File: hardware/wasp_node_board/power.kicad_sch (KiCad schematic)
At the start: 29 parts, among them J1 Conn_01x02, J7 USB_C_Receptacle_USB2.0_16P, SW1 C&K JS102011SAQN, U2 USBLC6-2SC6, U4 TPSM863253RDXR, U6 LP5907MFX-1.2

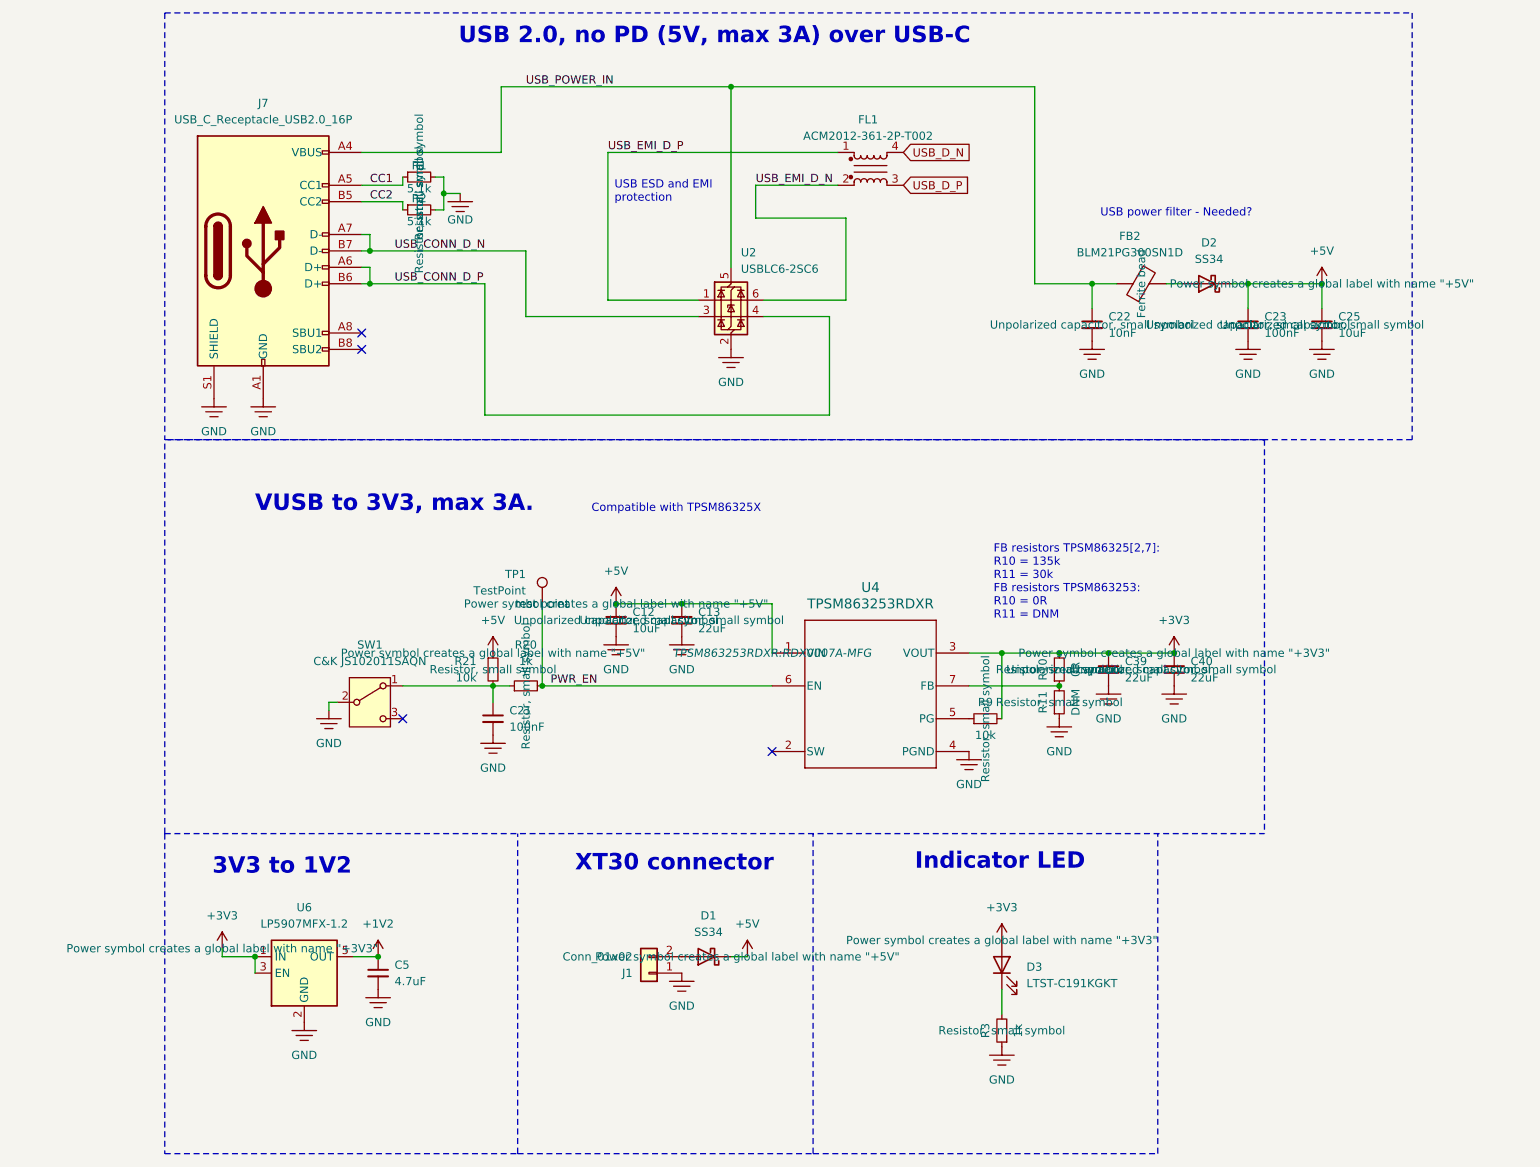
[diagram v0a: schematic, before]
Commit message: V1 layout done
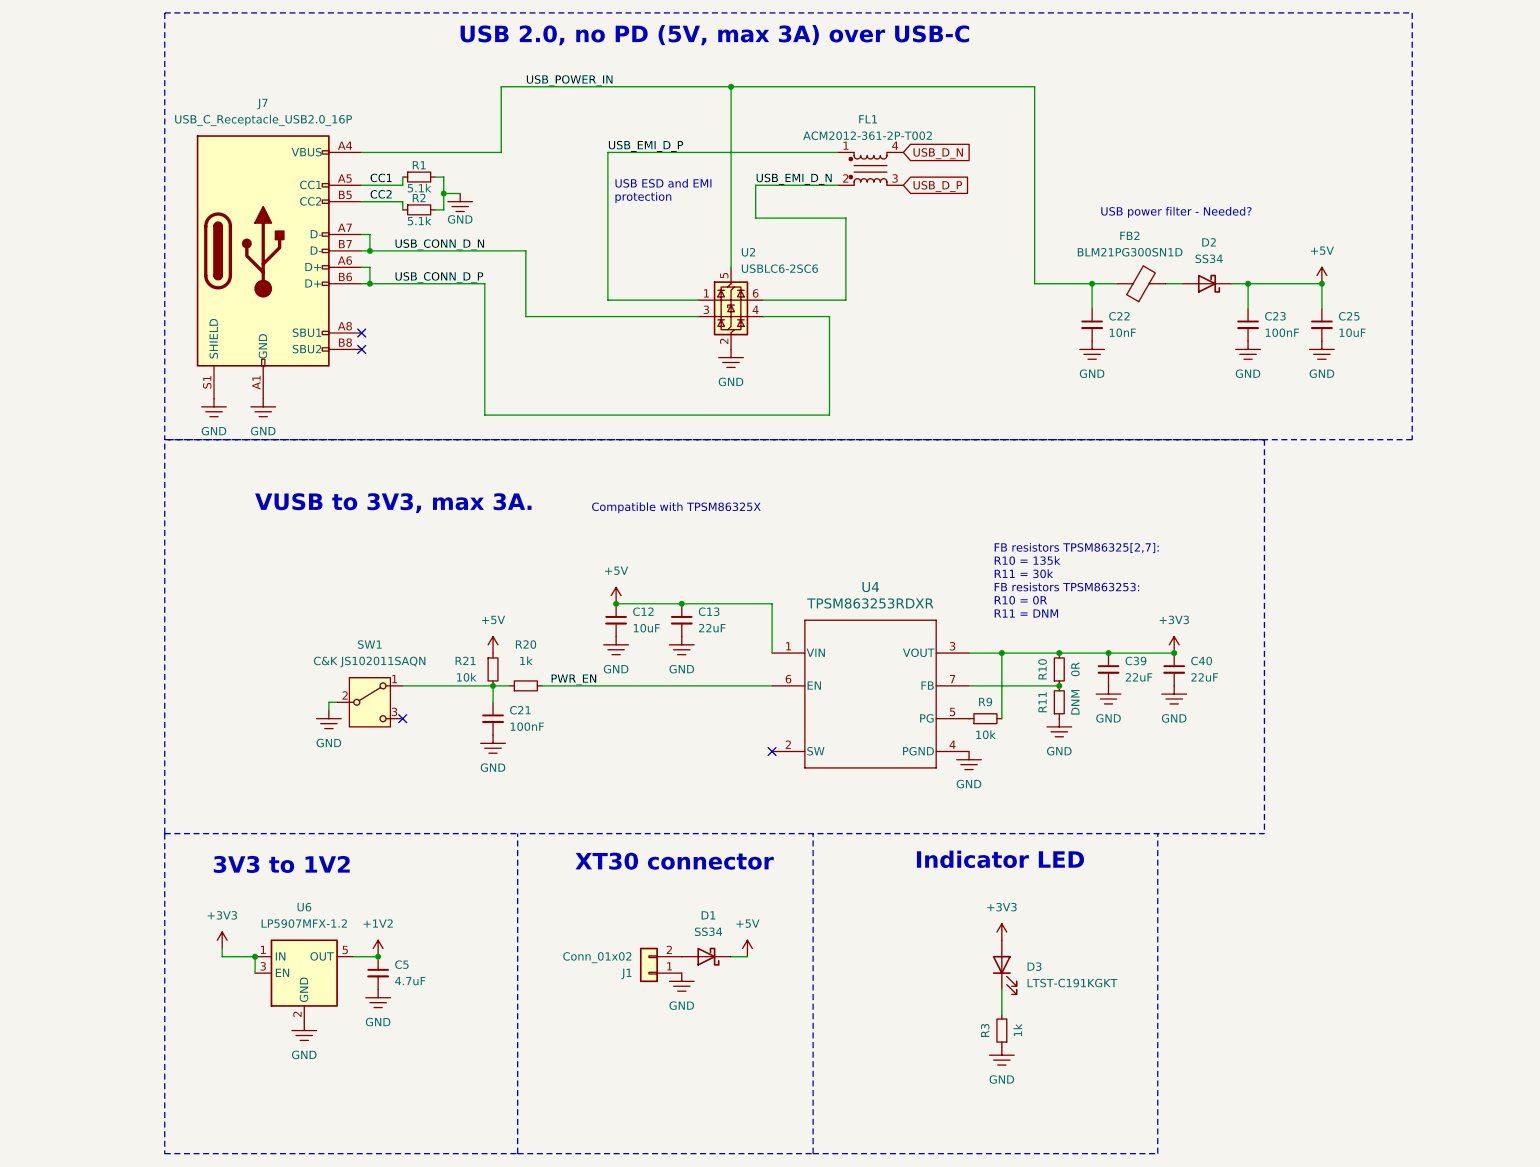
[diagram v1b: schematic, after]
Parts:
- removed TP1: TestPoint, TestPoint:TestPoint_Pad_1.0x1.0mm, symbol Connector:TestPoint
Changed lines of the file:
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@@
 	)
 	(junction
-		(at 76.2 118.11)
-		(diameter 0)
-		(color 0 0 0 0)
-	)
-	(junction
 		(at 31.75 160.02)
 		(diameter 0)
@@
 	(wire
 		(pts
-			(xy 76.2 105.41) (xy 76.2 118.11)
-		)
-		(stroke
-			(width 0)
-			(type default)
-		)
-	)
-	(wire
-		(pts
 			(xy 49.53 48.26) (xy 48.26 48.26)
 		)
@@
 					(size 1.27 1.27)
 				)
+				(hide yes)
 			)
 		)
@@
 					(size 1.27 1.27)
 				)
+				(hide yes)
 			)
 		)
@@
 					(size 1.27 1.27)
 				)
+				(hide yes)
 			)
 		)
@@
 					(size 1.27 1.27)
 				)
+				(hide yes)
 			)
 		)
@@
 					(size 1.27 1.27)
 				)
+				(hide yes)
 			)
 		)
@@
 					(size 1.27 1.27)
 				)
+				(hide yes)
 			)
 		)
@@
 					(size 1.27 1.27)
 				)
+				(hide yes)
 			)
 		)
@@
 					(size 1.27 1.27)
 				)
+				(hide yes)
 			)
 		)
@@
 					(size 1.27 1.27)
 				)
+				(hide yes)
 			)
 		)
@@
 					(size 1.27 1.27)
 				)
+				(hide yes)
 			)
 		)
@@
 					(size 1.27 1.27)
 				)
+				(hide yes)
 			)
 		)
@@
 					(size 1.27 1.27)
 				)
+				(hide yes)
 			)
 		)
@@
 					(size 1.27 1.27)
 				)
+				(hide yes)
 			)
 		)
@@
 					(size 1.27 1.27)
 				)
+				(hide yes)
 			)
 		)
@@
 					(size 1.27 1.27)
 				)
+				(hide yes)
 			)
 		)
@@
 					(size 1.27 1.27)
 				)
+				(hide yes)
 			)
 		)
@@
 					(italic yes)
 				)
+				(hide yes)
 			)
 		)
@@
 					(size 1.27 1.27)
 				)
+				(hide yes)
 			)
 		)
@@
 					(size 1.27 1.27)
 				)
+				(hide yes)
 			)
 		)
@@
 					(size 1.27 1.27)
 				)
+				(hide yes)
 			)
 		)
@@
 					(size 1.27 1.27)
 				)
+				(hide yes)
 			)
 		)
@@
 					(size 1.27 1.27)
 				)
+				(hide yes)
 			)
 		)
@@
 					(size 1.27 1.27)
 				)
+				(hide yes)
 			)
 		)
@@
 	)
 	(symbol
-		(lib_id "Connector:TestPoint")
-		(at 76.2 105.41 0)
-		(mirror y)
-		(unit 1)
-		(exclude_from_sim no)
-		(in_bom yes)
-		(on_board yes)
-		(dnp no)
-		(fields_autoplaced yes)
-		(property "Reference" "TP1"
-			(at 73.66 100.8379 0)
-			(effects
-				(font
-					(size 1.27 1.27)
-				)
-				(justify left)
-			)
-		)
-		(property "Value" "TestPoint"
-			(at 73.66 103.3779 0)
-			(effects
-				(font
-					(size 1.27 1.27)
-				)
-				(justify left)
-			)
-		)
-		(property "Footprint" "TestPoint:TestPoint_Pad_1.0x1.0mm"
-			(at 71.12 105.41 0)
-			(effects
-				(font
-					(size 1.27 1.27)
-				)
-				(hide yes)
-			)
-		)
-		(property "Datasheet" "~"
-			(at 71.12 105.41 0)
-			(effects
-				(font
-					(size 1.27 1.27)
-				)
-				(hide yes)
-			)
-		)
-		(property "Description" "test point"
-			(at 76.2 105.41 0)
-			(effects
-				(font
-					(size 1.27 1.27)
-				)
-			)
-		)
-		(pin "1"
-		)
-		(instances
-			(project "wasp_node_board"
-				(path "/8112a7f8-6a52-4f6e-80c5-c0e3be484a00/84c5fa1f-c7c3-4e8a-aae5-80440cd36d77"
-					(reference "TP1")
-					(unit 1)
-				)
-			)
-		)
-	)
-	(symbol
 		(lib_id "power:+5V")
 		(at 68.58 113.03 0)
@@
 					(size 1.27 1.27)
 				)
+				(hide yes)
 			)
 		)
